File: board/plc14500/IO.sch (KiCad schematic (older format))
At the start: 94 parts, among them U1 74HC14, U2 4051, U3 74HC14, U4 NE555, U5 Arduino Nano, U6 CD4099

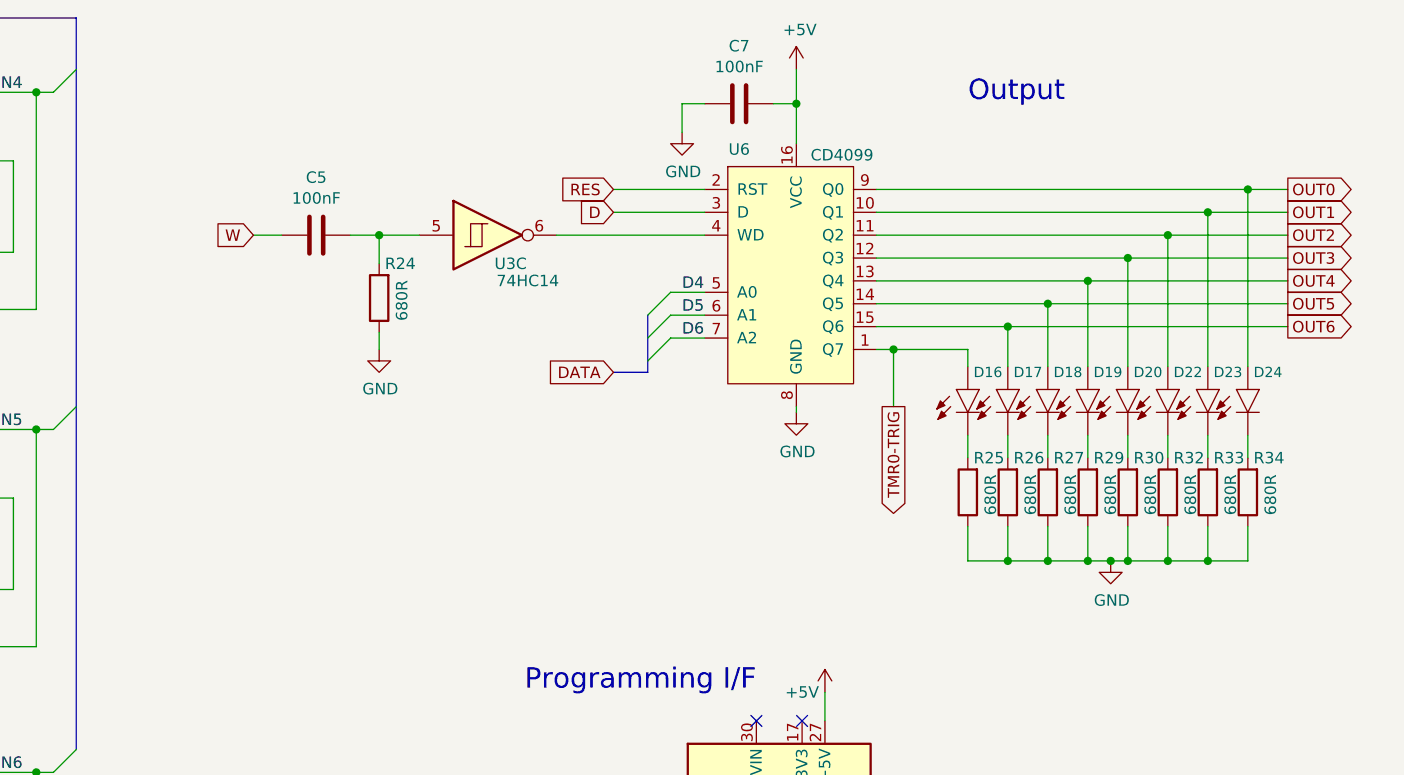
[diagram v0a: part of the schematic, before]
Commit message: Add assembler skeleton
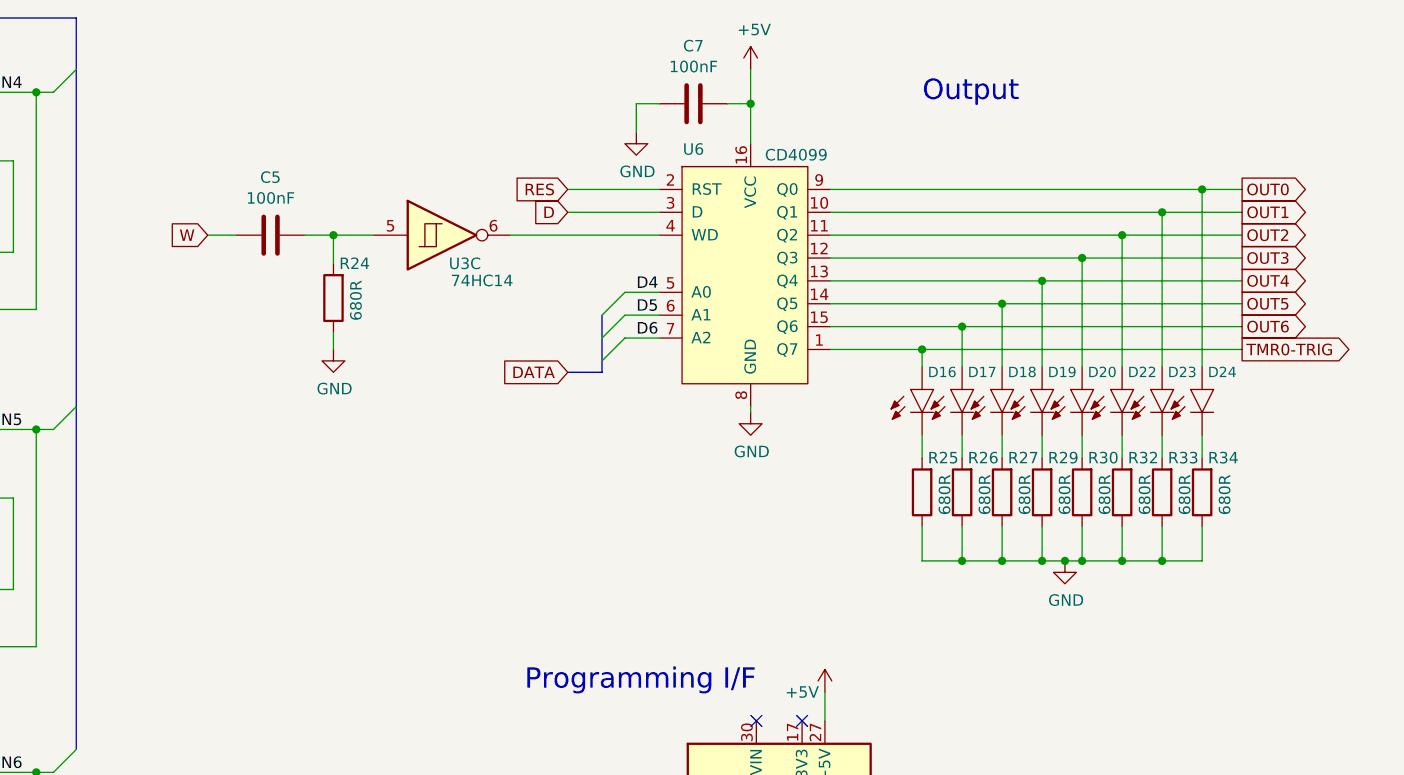
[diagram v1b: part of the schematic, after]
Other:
- moved on the sheet: C5, C7, D16, D17, D18, D19, D20, D22, D23, D24, R24, R25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
